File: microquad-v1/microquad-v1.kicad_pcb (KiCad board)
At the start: 2 copper layers, 83.8 x 74.3 mm, 79 parts, among them J1 USB_microB_2040002-1, M1 Motor_DC, M2 Motor_DC, M3 Motor_DC, M4 Motor_DC, M5 Motor_DC, M6 Motor_DC, Q1 Q_NMOS_GSD, Q2 Q_NMOS_GSD, Q3 Q_NMOS_GSD, Q4 Q_NMOS_GSD, Q5 Q_NMOS_GSD, Q6 Q_NMOS_GSD, SW1 SERIAL, SW2 POWER, SW3 RESET, U1 ATMEGA328PB, U2 MCP1703A-3302_SOT23, U3 FT230XS, U4 MCP73812T, U5 MAX6333UR18D3

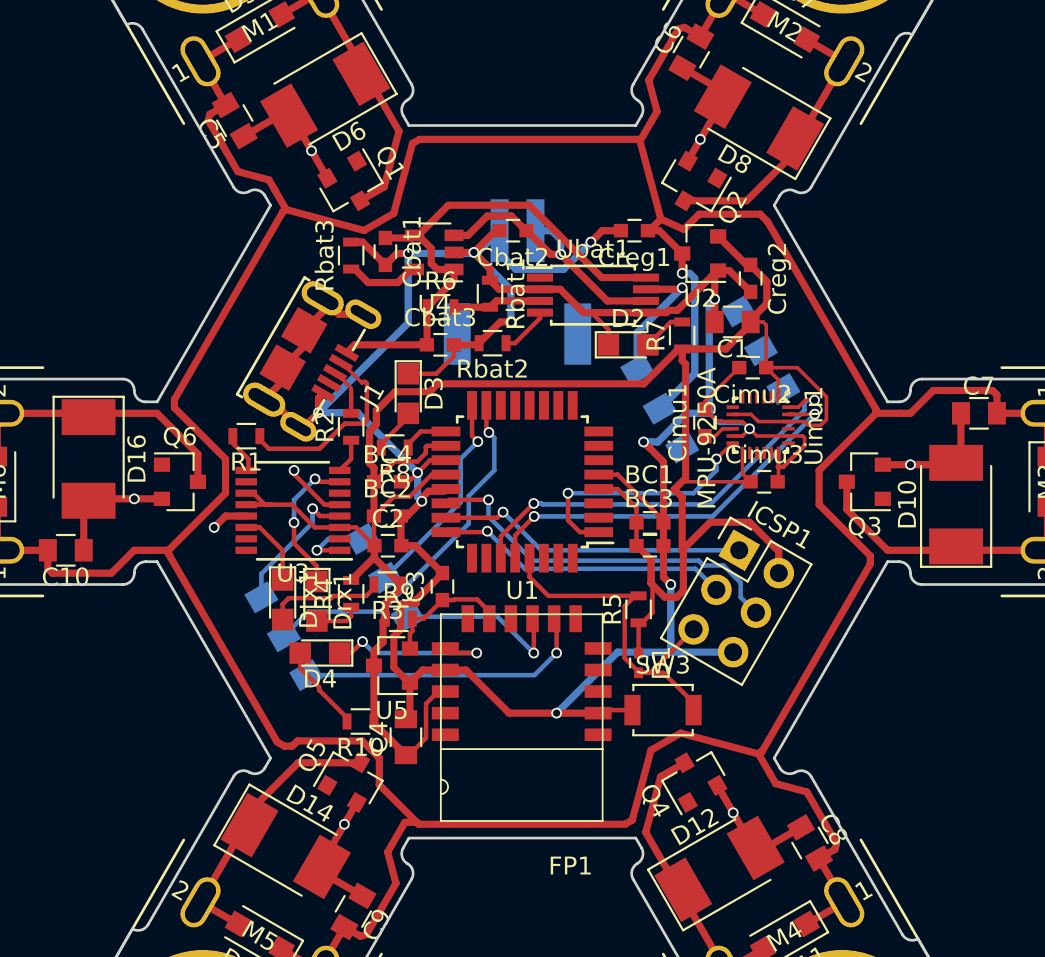
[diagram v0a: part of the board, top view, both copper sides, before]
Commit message: Ladybug is satisfied
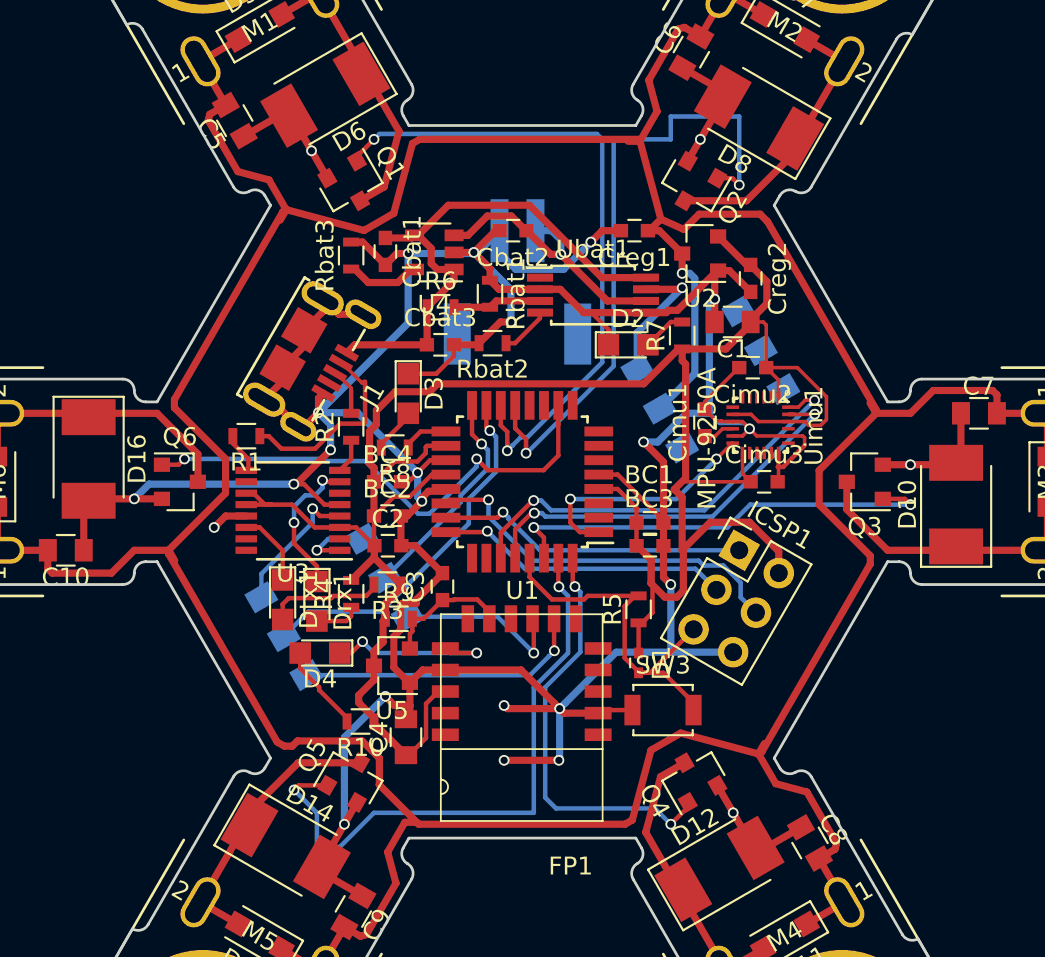
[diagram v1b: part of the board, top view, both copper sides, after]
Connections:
- U1 pad 13: /Motor5/ENABLE -> /Motor2/ENABLE
- U1 pad 14: /Motor4/ENABLE -> /Motor1/ENABLE
- U1 pad 31: /Motor2/ENABLE -> /Motor5/ENABLE
- U1 pad 32: /Motor1/ENABLE -> /Motor4/ENABLE
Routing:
- net /Motor1/ENABLE: track 0.00 -> 37.0 mm, vias 0 -> 2
- net /Motor2/ENABLE: track 0.00 -> 35.8 mm, vias 0 -> 2
- net /Motor5/ENABLE: track 0.00 -> 33.7 mm, vias 0 -> 2
- net GND: track 229.0 -> 261.5 mm, vias 20 -> 25
- net /Motor6/ENABLE: track 0.00 -> 28.3 mm, vias 0 -> 2
- net /Motor3/ENABLE: track 0.00 -> 25.1 mm, vias 0 -> 2
- net /Motor4/ENABLE: track 0.00 -> 23.5 mm, vias 0 -> 2
- net /VBAT: track 234.5 -> 237.6 mm
- net /IMU_INT: track 14.2 -> 13.4 mm
- net +3V3: track 137.7 -> 138.4 mm
